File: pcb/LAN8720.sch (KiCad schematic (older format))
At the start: 23 parts, among them J15 RJ45_Amphenol_RJMG1BD3B8K1ANR, U11 LAN8720A

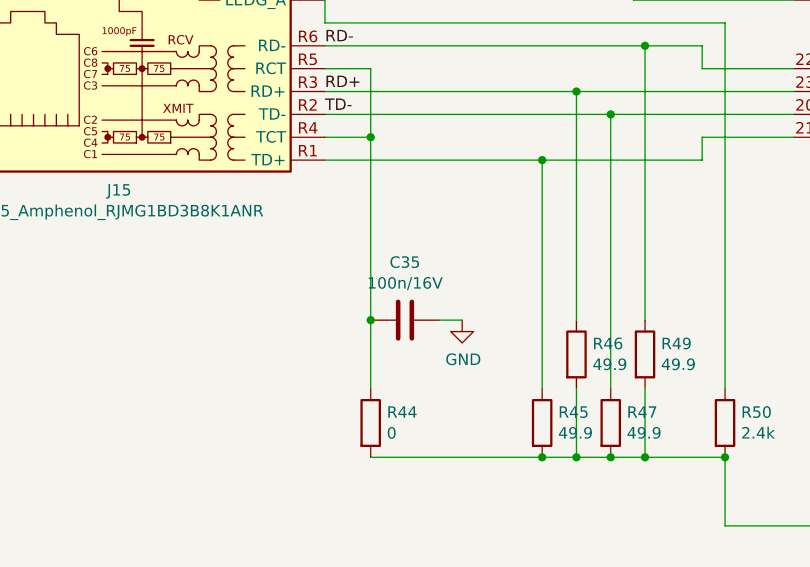
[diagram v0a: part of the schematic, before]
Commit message: chage LED footprint(D2,D5,D9)
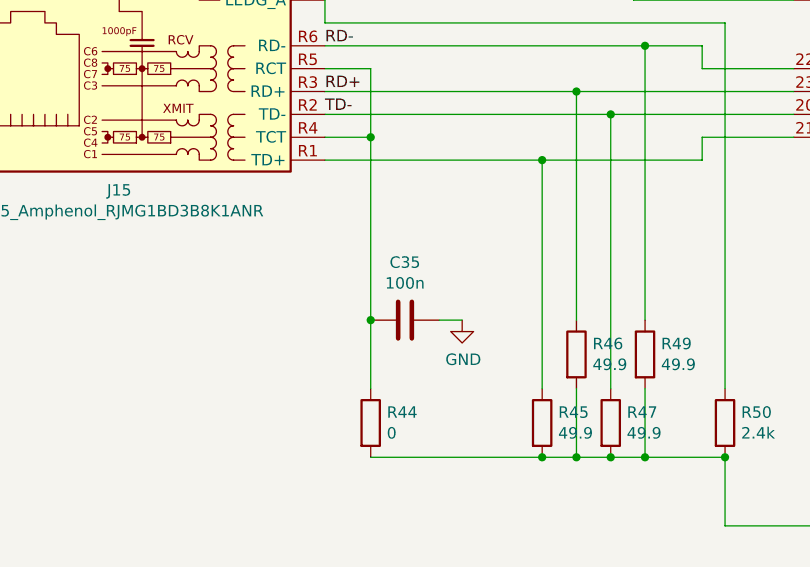
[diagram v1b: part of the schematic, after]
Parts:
- C35: value 100n/16V -> 100n
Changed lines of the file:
@@
 EESchema Schematic File Version 4
 LIBS:mainPCB-cache
-EELAYER 26 0
+EELAYER 29 0
 EELAYER END
 $Descr A4 11693 8268
@@
 P 2900 4650
 F 0 "C35" V 2648 4650 50  0000 C CNN
-F 1 "100n/16V" V 2739 4650 50  0000 C CNN
+F 1 "100n" V 2739 4650 50  0000 C CNN
 F 2 "Capacitor_SMD:C_0805_2012Metric" H 2938 4500 50  0001 C CNN
 F 3 "~" H 2900 4650 50  0001 C CNN

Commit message: reset code
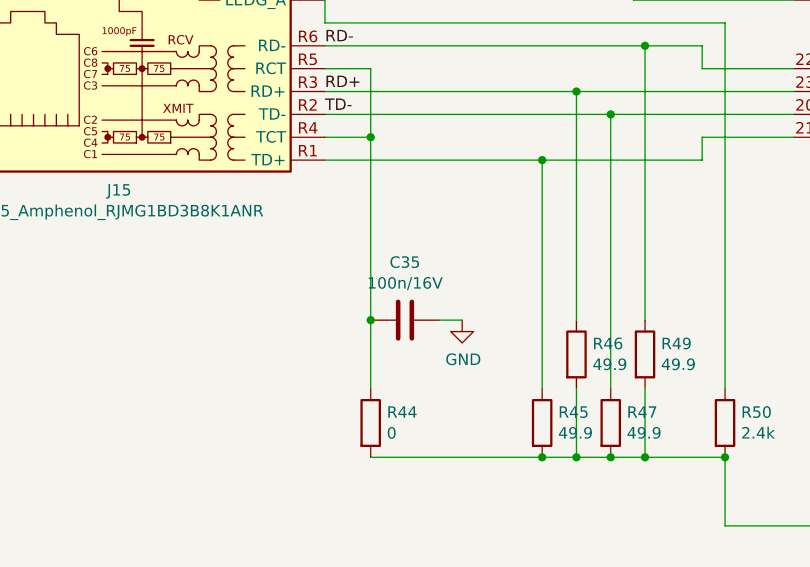
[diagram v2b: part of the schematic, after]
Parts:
- C35: value 100n -> 100n/16V
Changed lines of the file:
@@
 EESchema Schematic File Version 4
 LIBS:mainPCB-cache
-EELAYER 29 0
+EELAYER 26 0
 EELAYER END
 $Descr A4 11693 8268
@@
 P 2900 4650
 F 0 "C35" V 2648 4650 50  0000 C CNN
-F 1 "100n" V 2739 4650 50  0000 C CNN
+F 1 "100n/16V" V 2739 4650 50  0000 C CNN
 F 2 "Capacitor_SMD:C_0805_2012Metric" H 2938 4500 50  0001 C CNN
 F 3 "~" H 2900 4650 50  0001 C CNN
